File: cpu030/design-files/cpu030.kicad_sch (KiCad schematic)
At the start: 71 parts, among them J101 Reset, J102 SYSCTL JTAG, J103 NMI, SW101 Reset, SW102 NMI, U101 MC68030, U102 ATF1508AS, U103 74ACT05, U104 DS1813, U105 SST39SF040 (E), U106 SST39SF040 (O), U107 MC68882, U108 GAL22V10, U109 74ACT05, U110 DS1813, Y101 50MHz

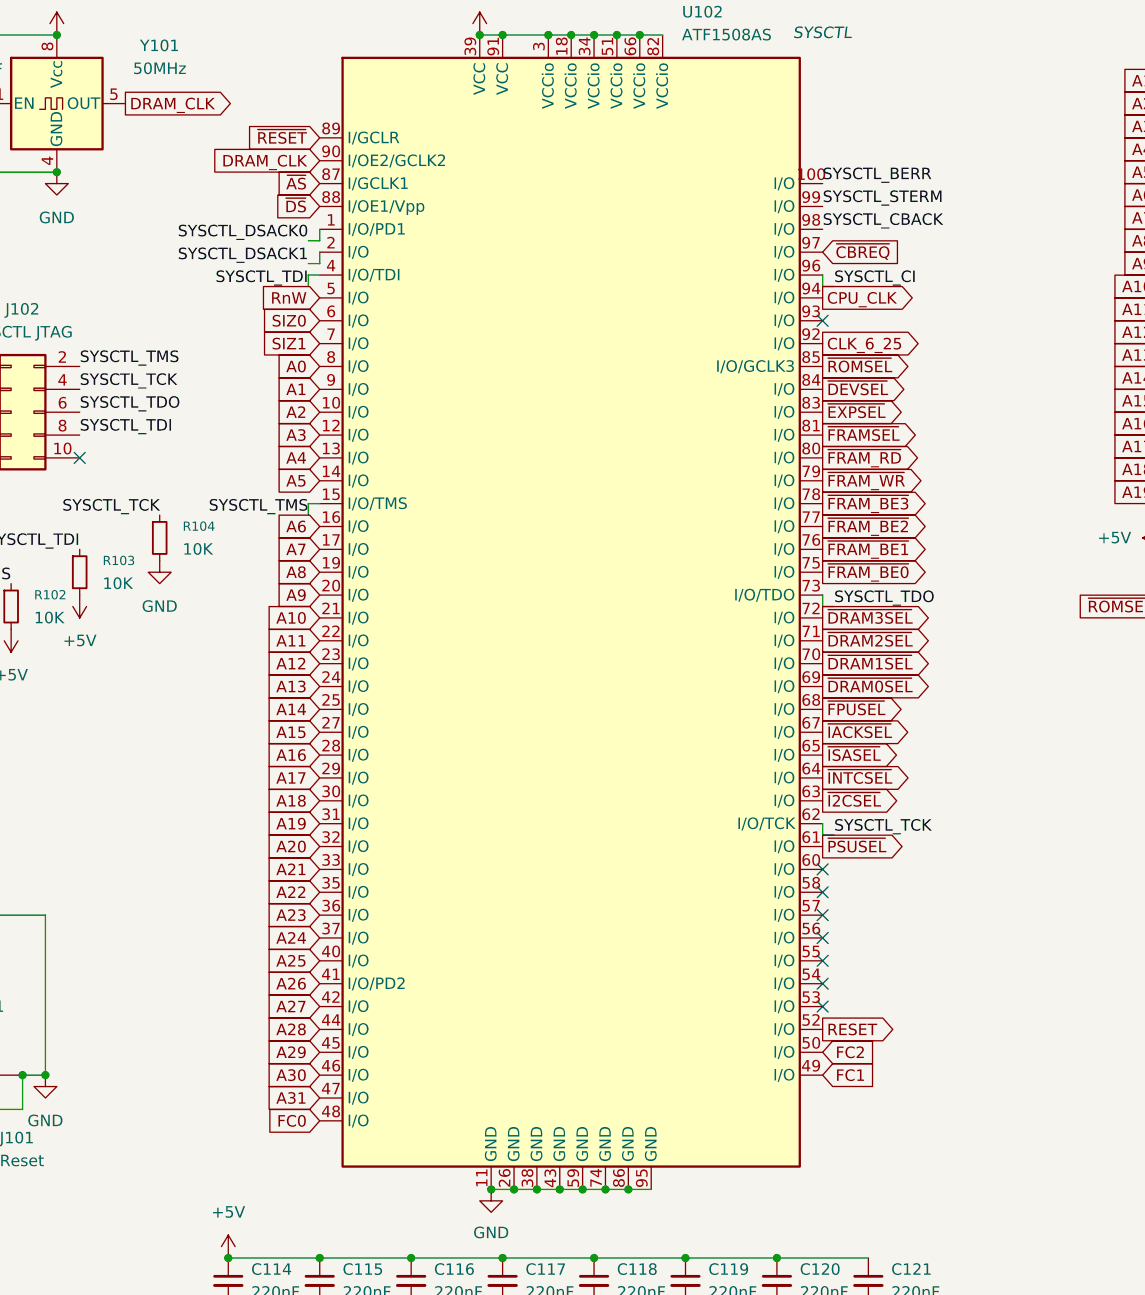
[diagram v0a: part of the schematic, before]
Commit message: Re-pin SYSCTL to make signal routing a lot easier.
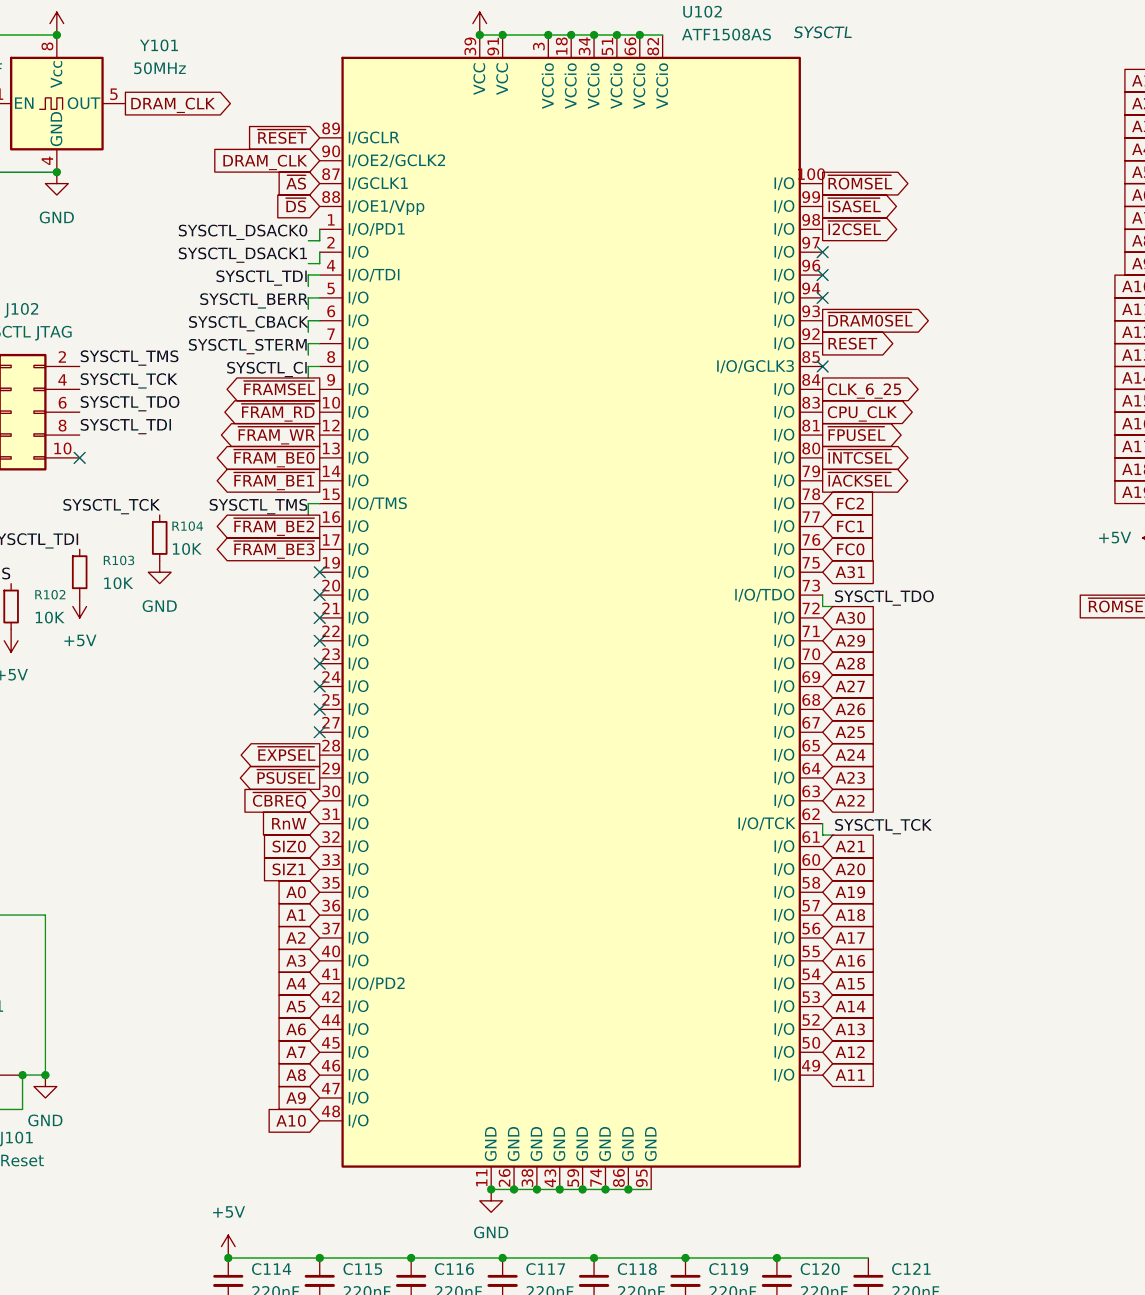
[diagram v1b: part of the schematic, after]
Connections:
- net ~{DEVSEL} is gone; now on net CLK_6_25: U102.84 (I/O)
- net ~{DRAM1SEL} is gone; now on net A28: U102.70 (I/O)
- net ~{DRAM2SEL} is gone; now on net A29: U102.71 (I/O)
- net ~{DRAM3SEL} is gone; now on net A30: U102.72 (I/O)
- net A0: now also U102.35 (I/O); no longer U102.8 (I/O)
- net A1: now also U102.36 (I/O); no longer U102.9 (I/O)
- net A10: now also U102.48 (I/O); no longer U102.21 (I/O)
- net A11: now also U102.49 (I/O); no longer U102.22 (I/O)
- net A12: now also U102.50 (I/O); no longer U102.23 (I/O)
- net A13: now also U102.52 (I/O); no longer U102.24 (I/O)
- net A14: now also U102.53 (I/O); no longer U102.25 (I/O)
- net A15: now also U102.54 (I/O); no longer U102.27 (I/O)
- net A16: now also U102.55 (I/O); no longer U102.28 (I/O)
- net A17: now also U102.56 (I/O); no longer U102.29 (I/O)
- net A18: now also U102.57 (I/O); no longer U102.30 (I/O)
- net A19: now also U102.58 (I/O); no longer U102.31 (I/O)
- net A2: now also U102.37 (I/O); no longer U102.10 (I/O)
- net A20: now also U102.60 (I/O); no longer U102.32 (I/O)
- net A21: now also U102.61 (I/O); no longer U102.33 (I/O)
- net A22: now also U102.63 (I/O); no longer U102.35 (I/O)
- net A23: now also U102.64 (I/O); no longer U102.36 (I/O)
- net A24: now also U102.65 (I/O); no longer U102.37 (I/O)
- net A25: now also U102.67 (I/O); no longer U102.40 (I/O)
- net A26: now also U102.68 (I/O); no longer U102.41 (I/O/PD2)
- net A27: now also U102.69 (I/O); no longer U102.42 (I/O)
- net A28: no longer U102.44 (I/O)
- net A29: no longer U102.45 (I/O)
- net A3: now also U102.40 (I/O); no longer U102.12 (I/O)
- net A30: no longer U102.46 (I/O)
- net A31: now also U102.75 (I/O); no longer U102.47 (I/O)
- net A4: now also U102.41 (I/O/PD2); no longer U102.13 (I/O)
- net A5: now also U102.42 (I/O); no longer U102.14 (I/O)
- net A6: now also U102.44 (I/O); no longer U102.16 (I/O)
- net A7: now also U102.45 (I/O); no longer U102.17 (I/O)
- net A8: now also U102.46 (I/O); no longer U102.19 (I/O)
- net A9: now also U102.47 (I/O); no longer U102.20 (I/O)
- net CLK_6_25: no longer U102.92 (I/O)
- net CPU_CLK: now also U102.83 (I/O); no longer U102.94 (I/O)
- net FC0: now also U102.76 (I/O); no longer U102.48 (I/O)
- net FC1: now also U102.77 (I/O); no longer U102.49 (I/O)
- net FC2: now also U102.78 (I/O); no longer U102.50 (I/O)
- net RESET: now also U102.92 (I/O); no longer U102.52 (I/O)
- net RnW: now also U102.31 (I/O); no longer U102.5 (I/O)
- net SIZ0: now also U102.32 (I/O); no longer U102.6 (I/O)
- net SIZ1: now also U102.33 (I/O); no longer U102.7 (I/O)
- net SYSCTL_BERR: now also U102.5 (I/O); no longer U102.100 (I/O)
- net SYSCTL_CBACK: now also U102.6 (I/O); no longer U102.98 (I/O)
- net SYSCTL_CI: now also U102.8 (I/O); no longer U102.96 (I/O)
- net SYSCTL_STERM: now also U102.7 (I/O); no longer U102.99 (I/O)
- net ~{CBREQ}: now also U102.30 (I/O); no longer U102.97 (I/O)
- net ~{DRAM0SEL}: now also U102.93 (I/O); no longer U102.69 (I/O)
- net ~{EXPSEL}: now also U102.28 (I/O); no longer U102.83 (I/O)
- net ~{FPUSEL}: now also U102.81 (I/O); no longer U102.68 (I/O)
- net ~{FRAMSEL}: now also U102.9 (I/O); no longer U102.81 (I/O)
- net ~{FRAM_BE0}: now also U102.13 (I/O); no longer U102.75 (I/O)
- net ~{FRAM_BE1}: now also U102.14 (I/O); no longer U102.76 (I/O)
- net ~{FRAM_BE2}: now also U102.16 (I/O); no longer U102.77 (I/O)
- net ~{FRAM_BE3}: now also U102.17 (I/O); no longer U102.78 (I/O)
- net ~{FRAM_RD}: now also U102.10 (I/O); no longer U102.80 (I/O)
- net ~{FRAM_WR}: now also U102.12 (I/O); no longer U102.79 (I/O)
- net ~{I2CSEL}: now also U102.98 (I/O); no longer U102.63 (I/O)
- net ~{IACKSEL}: now also U102.79 (I/O); no longer U102.67 (I/O)
- net ~{INTCSEL}: now also U102.80 (I/O); no longer U102.64 (I/O)
- net ~{ISASEL}: now also U102.99 (I/O); no longer U102.65 (I/O)
- net ~{PSUSEL}: now also U102.29 (I/O); no longer U102.61 (I/O)
- net ~{ROMSEL}: now also U102.100 (I/O); no longer U102.85 (I/O/GCLK3)
- no-connect marks 25 -> 29
